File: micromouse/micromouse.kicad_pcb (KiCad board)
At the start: 2 copper layers, 128.6 x 114.7 mm, 81 parts, among them IC1 STM32F205RET7, J1 B2B-PH-K-S, J2 B2B-PH-K-S, J3 Left Header, J4 Left Header, J5 Conn_01x04_Pin, Q1 ir_reciever, Q2 ir_reciever, Q3 SFH_313_FA-3_4, Q4 SFH_313_FA-3_4, Q5 2N7002LT1G, Q6 2N7002LT1G, Q7 2N7002LT1G, Q8 2N7002LT1G, SW1 CK_KMS2xxG, SW2 EG1218, U2 AZ1117IH-3.3TRG1, U3 L293DD, U5 LSM6DSOTR

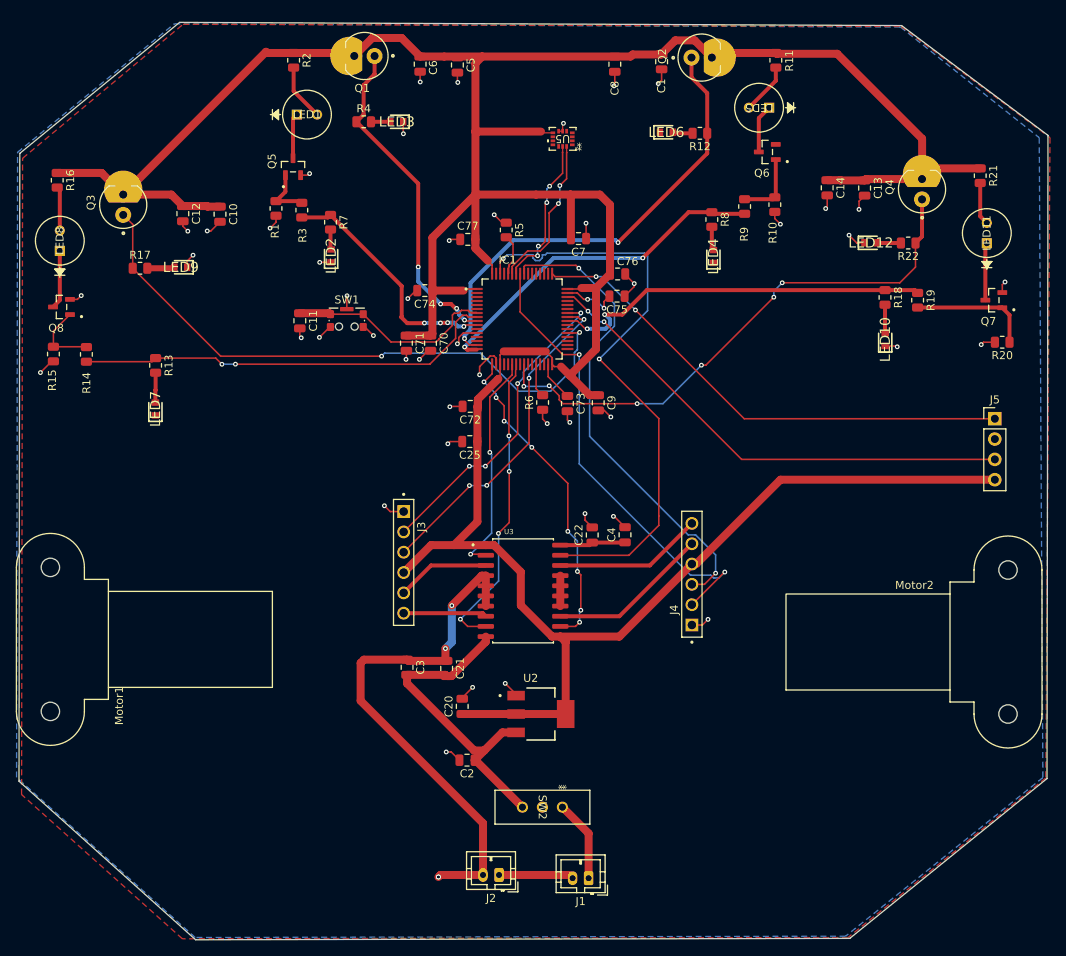
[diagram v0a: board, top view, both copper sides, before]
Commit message: final
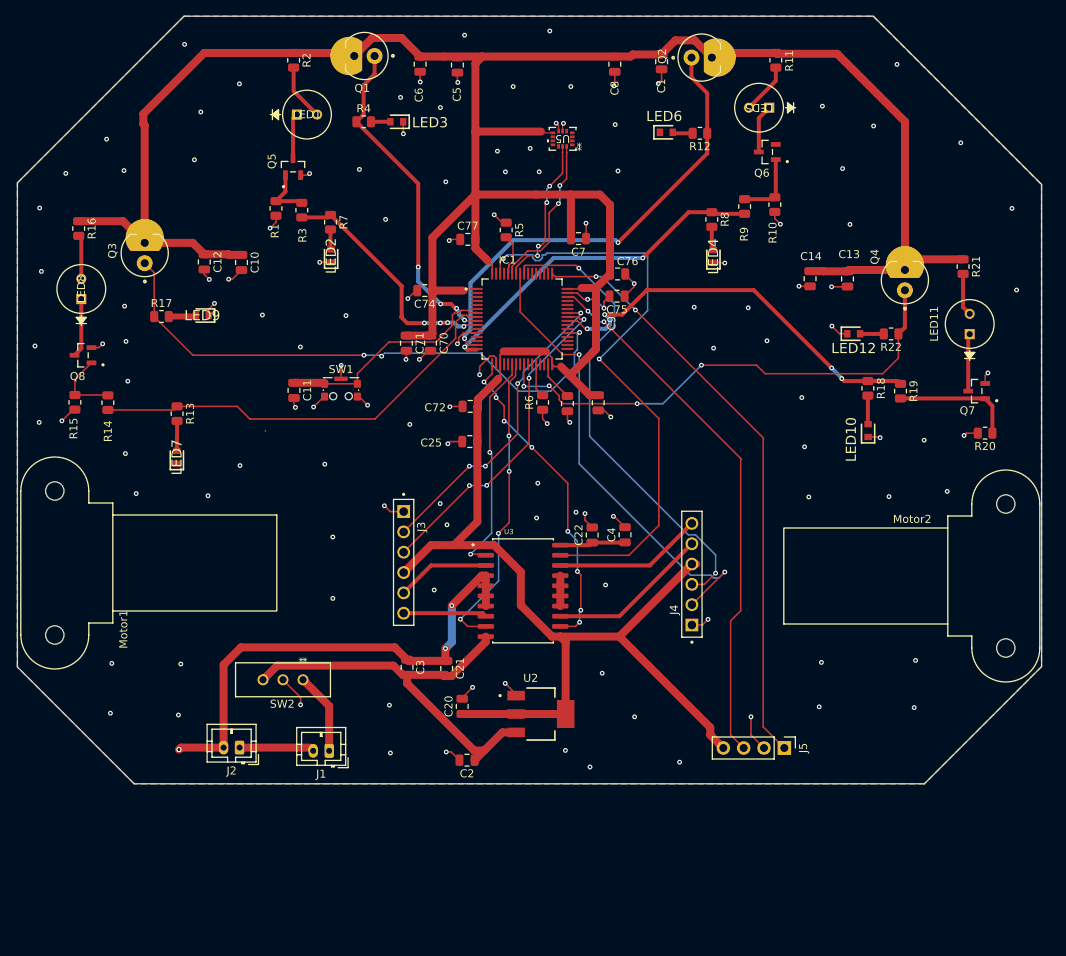
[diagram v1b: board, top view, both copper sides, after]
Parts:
- C73: value 2.2uF -> C2.2uF
- C9: value 0.1 uF -> C0.1 uF
- J1, J2: value B2B-PH-K-S -> Battery Conn
- J4: value Left Header -> Right Header
- J5: value Conn_01x04_Pin -> Debug Pins
- LED1, LED11, LED5, LED8: value INL-5AMIR15 -> ir reciever
- Q1, Q2: value ir_reciever -> ir_emitter
- Q3, Q4: value SFH_313_FA-3_4 -> ir emmiter
- Q5, Q6, Q7, Q8: value 2N7002LT1G -> mosfet
- SW1: value CK_KMS2xxG -> reset switch
- SW2: value EG1218 -> Switch
- U2: value AZ1117IH-3.3TRG1 -> Voltage Regulator
- U5: value LSM6DSOTR -> gyro/accel
- moved J5 48.8 mm to (133.2, 108.4), turned to -90 degrees
- moved J1 36.1 mm to (76.3, 108.7)
- moved J2 36.1 mm to (65.2, 108.3)
- moved SW2 36.1 mm to (73.1, 99.8)
- moved C13 11.6 mm to (141.1, 49.7)
- moved LED12 11.6 mm to (141.9, 56.6)
- moved Q7 11.6 mm to (157.3, 63.8)
- moved C14 11.6 mm to (136.5, 49.7)
- moved LED11 11.6 mm to (156.4, 56.6)
- moved R19 11.6 mm to (147.8, 63.8)
- moved R21 11.6 mm to (155.6, 48.2)
- moved R22 11.6 mm to (146.6, 56.6)
- moved LED10 11.6 mm to (143.7, 68.7)
- moved Q4 11.6 mm to (148.3, 49.9)
- moved R18 11.6 mm to (143.7, 63.4)
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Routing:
- net SWCLK: track 62.9 -> 74.8 mm
- net VCC: track 49.8 -> 60.7 mm
- net GND: track 88.1 -> 98.4 mm, vias 48 -> 131
- net PC5: track 69.3 -> 62.9 mm, vias 6 -> 4
- net SWDIO: track 61.8 -> 67.6 mm
- net PC6: track 76.5 -> 71.3 mm, vias 2 -> 3
- net MGND: track 70.2 -> 66.2 mm
- net PC9: track 48.0 -> 50.6 mm, vias 2 -> 4
- net 3V3: track 434.5 -> 432.0 mm
- net NRST: track 26.2 -> 28.4 mm
- net PC0: track 53.1 -> 53.6 mm, vias 2 -> 0
- net (no net): vias 0 -> 1
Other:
- board size 128.6 x 114.7 mm -> 128 x 95.9 mm
